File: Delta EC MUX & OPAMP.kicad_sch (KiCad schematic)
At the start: 32 parts, among them U6 OPA2365, U7 4052, U8 OPA2365, U9 4052

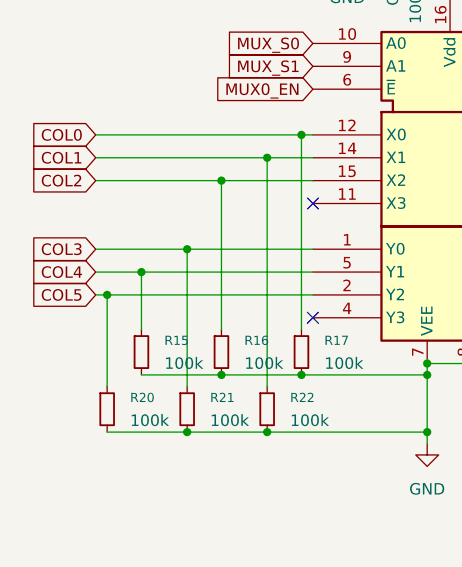
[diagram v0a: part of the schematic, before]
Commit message: 17.04.2026
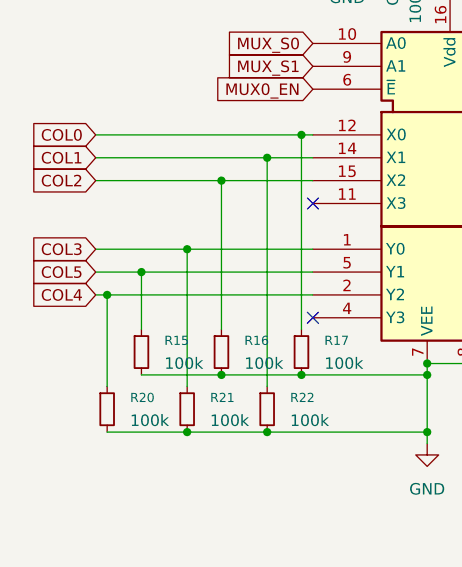
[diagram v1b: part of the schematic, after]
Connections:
- net COL4: now also R20.1, U7.2 (Y2); no longer R15.1, U7.5 (Y1)
- net COL5: now also R15.1, U7.5 (Y1); no longer R20.1, U7.2 (Y2)
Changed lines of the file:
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@@
 	(global_label "COL4"
 		(shape input)
+		(at 40.64 74.93 180)
+		(fields_autoplaced yes)
+		(effects
+			(font
+				(size 1.27 1.27)
+			)
+			(justify right)
+		)
+		(property "Intersheetrefs" "${INTERSHEET_REFS}"
+			(at 32.8167 74.93 0)
+			(effects
+				(font
+					(size 1.27 1.27)
+				)
+				(justify right)
+				(hide yes)
+			)
+		)
+	)
+	(global_label "COL3"
+		(shape input)
+		(at 40.64 69.85 180)
+		(fields_autoplaced yes)
+		(effects
+			(font
+				(size 1.27 1.27)
+			)
+			(justify right)
+		)
+		(property "Intersheetrefs" "${INTERSHEET_REFS}"
+			(at 32.8167 69.85 0)
+			(effects
+				(font
+					(size 1.27 1.27)
+				)
+				(justify right)
+				(hide yes)
+			)
+		)
+	)
+	(global_label "ADC2_IN"
+		(shape input)
+		(at 139.7 132.08 0)
+		(fields_autoplaced yes)
+		(effects
+			(font
+				(size 1.27 1.27)
+			)
+			(justify left)
+		)
+		(property "Intersheetrefs" "${INTERSHEET_REFS}"
+			(at 150.4262 132.08 0)
+			(effects
+				(font
+					(size 1.27 1.27)
+				)
+				(justify left)
+				(hide yes)
+			)
+		)
+	)
+	(global_label "ADC1_IN"
+		(shape input)
+		(at 119.38 76.2 0)
+		(fields_autoplaced yes)
+		(effects
+			(font
+				(size 1.27 1.27)
+			)
+			(justify left)
+		)
+		(property "Intersheetrefs" "${INTERSHEET_REFS}"
+			(at 130.1062 76.2 0)
+			(effects
+				(font
+					(size 1.27 1.27)
+				)
+				(justify left)
+				(hide yes)
+			)
+		)
+	)
+	(global_label "COL10"
+		(shape input)
+		(at 48.26 157.48 180)
+		(fields_autoplaced yes)
+		(effects
+			(font
+				(size 1.27 1.27)
+			)
+			(justify right)
+		)
+		(property "Intersheetrefs" "${INTERSHEET_REFS}"
+			(at 39.2272 157.48 0)
+			(effects
+				(font
+					(size 1.27 1.27)
+				)
+				(justify right)
+				(hide yes)
+			)
+		)
+	)
+	(global_label "COL1"
+		(shape input)
+		(at 40.64 59.69 180)
+		(fields_autoplaced yes)
+		(effects
+			(font
+				(size 1.27 1.27)
+			)
+			(justify right)
+		)
+		(property "Intersheetrefs" "${INTERSHEET_REFS}"
+			(at 32.8167 59.69 0)
+			(effects
+				(font
+					(size 1.27 1.27)
+				)
+				(justify right)
+				(hide yes)
+			)
+		)
+	)
+	(global_label "DISCHARGE0"
+		(shape input)
+		(at 104.14 43.18 90)
+		(fields_autoplaced yes)
+		(effects
+			(font
+				(size 1.27 1.27)
+			)
+			(justify left)
+		)
+		(property "Intersheetrefs" "${INTERSHEET_REFS}"
+			(at 104.14 28.5229 90)
+			(effects
+				(font
+					(size 1.27 1.27)
+				)
+				(justify left)
+				(hide yes)
+			)
+		)
+	)
+	(global_label "COL7"
+		(shape input)
+		(at 48.26 144.78 180)
+		(fields_autoplaced yes)
+		(effects
+			(font
+				(size 1.27 1.27)
+			)
+			(justify right)
+		)
+		(property "Intersheetrefs" "${INTERSHEET_REFS}"
+			(at 40.4367 144.78 0)
+			(effects
+				(font
+					(size 1.27 1.27)
+				)
+				(justify right)
+				(hide yes)
+			)
+		)
+	)
+	(global_label "MUX_S1"
+		(shape input)
+		(at 64.77 49.53 180)
+		(fields_autoplaced yes)
+		(effects
+			(font
+				(size 1.27 1.27)
+			)
+			(justify right)
+		)
+		(property "Intersheetrefs" "${INTERSHEET_REFS}"
+			(at 54.4068 49.53 0)
+			(effects
+				(font
+					(size 1.27 1.27)
+				)
+				(justify right)
+				(hide yes)
+			)
+		)
+	)
+	(global_label "DISCHARGE2"
+		(shape input)
+		(at 111.76 128.27 90)
+		(fields_autoplaced yes)
+		(effects
+			(font
+				(size 1.27 1.27)
+			)
+			(justify left)
+		)
+		(property "Intersheetrefs" "${INTERSHEET_REFS}"
+			(at 111.76 113.6129 90)
+			(effects
+				(font
+					(size 1.27 1.27)
+				)
+				(justify left)
+				(hide yes)
+			)
+		)
+	)
+	(global_label "DISCHARGE3"
+		(shape input)
+		(at 105.41 157.48 90)
+		(fields_autoplaced yes)
+		(effects
+			(font
+				(size 1.27 1.27)
+			)
+			(justify left)
+		)
+		(property "Intersheetrefs" "${INTERSHEET_REFS}"
+			(at 105.41 142.8229 90)
+			(effects
+				(font
+					(size 1.27 1.27)
+				)
+				(justify left)
+				(hide yes)
+			)
+		)
+	)
+	(global_label "COL5"
+		(shape input)
 		(at 40.64 72.39 180)
 		(fields_autoplaced yes)
@@
 			(effects
 				(font
-					(size 1.27 1.27)
-				)
-				(justify right)
-				(hide yes)
-			)
-		)
-	)
-	(global_label "COL3"
-		(shape input)
-		(at 40.64 69.85 180)
-		(fields_autoplaced yes)
-		(effects
-			(font
-				(size 1.27 1.27)
-			)
-			(justify right)
-		)
-		(property "Intersheetrefs" "${INTERSHEET_REFS}"
-			(at 32.8167 69.85 0)
-			(effects
-				(font
-					(size 1.27 1.27)
-				)
-				(justify right)
-				(hide yes)
-			)
-		)
-	)
-	(global_label "ADC2_IN"
-		(shape input)
-		(at 139.7 132.08 0)
-		(fields_autoplaced yes)
-		(effects
-			(font
-				(size 1.27 1.27)
-			)
-			(justify left)
-		)
-		(property "Intersheetrefs" "${INTERSHEET_REFS}"
-			(at 150.4262 132.08 0)
-			(effects
-				(font
-					(size 1.27 1.27)
-				)
-				(justify left)
-				(hide yes)
-			)
-		)
-	)
-	(global_label "ADC1_IN"
-		(shape input)
-		(at 119.38 76.2 0)
-		(fields_autoplaced yes)
-		(effects
-			(font
-				(size 1.27 1.27)
-			)
-			(justify left)
-		)
-		(property "Intersheetrefs" "${INTERSHEET_REFS}"
-			(at 130.1062 76.2 0)
-			(effects
-				(font
-					(size 1.27 1.27)
-				)
-				(justify left)
-				(hide yes)
-			)
-		)
-	)
-	(global_label "COL10"
-		(shape input)
-		(at 48.26 157.48 180)
-		(fields_autoplaced yes)
-		(effects
-			(font
-				(size 1.27 1.27)
-			)
-			(justify right)
-		)
-		(property "Intersheetrefs" "${INTERSHEET_REFS}"
-			(at 39.2272 157.48 0)
-			(effects
-				(font
-					(size 1.27 1.27)
-				)
-				(justify right)
-				(hide yes)
-			)
-		)
-	)
-	(global_label "COL1"
-		(shape input)
-		(at 40.64 59.69 180)
-		(fields_autoplaced yes)
-		(effects
-			(font
-				(size 1.27 1.27)
-			)
-			(justify right)
-		)
-		(property "Intersheetrefs" "${INTERSHEET_REFS}"
-			(at 32.8167 59.69 0)
-			(effects
-				(font
-					(size 1.27 1.27)
-				)
-				(justify right)
-				(hide yes)
-			)
-		)
-	)
-	(global_label "DISCHARGE0"
-		(shape input)
-		(at 104.14 43.18 90)
-		(fields_autoplaced yes)
-		(effects
-			(font
-				(size 1.27 1.27)
-			)
-			(justify left)
-		)
-		(property "Intersheetrefs" "${INTERSHEET_REFS}"
-			(at 104.14 28.5229 90)
-			(effects
-				(font
-					(size 1.27 1.27)
-				)
-				(justify left)
-				(hide yes)
-			)
-		)
-	)
-	(global_label "COL7"
-		(shape input)
-		(at 48.26 144.78 180)
-		(fields_autoplaced yes)
-		(effects
-			(font
-				(size 1.27 1.27)
-			)
-			(justify right)
-		)
-		(property "Intersheetrefs" "${INTERSHEET_REFS}"
-			(at 40.4367 144.78 0)
-			(effects
-				(font
-					(size 1.27 1.27)
-				)
-				(justify right)
-				(hide yes)
-			)
-		)
-	)
-	(global_label "MUX_S1"
-		(shape input)
-		(at 64.77 49.53 180)
-		(fields_autoplaced yes)
-		(effects
-			(font
-				(size 1.27 1.27)
-			)
-			(justify right)
-		)
-		(property "Intersheetrefs" "${INTERSHEET_REFS}"
-			(at 54.4068 49.53 0)
-			(effects
-				(font
-					(size 1.27 1.27)
-				)
-				(justify right)
-				(hide yes)
-			)
-		)
-	)
-	(global_label "DISCHARGE2"
-		(shape input)
-		(at 111.76 128.27 90)
-		(fields_autoplaced yes)
-		(effects
-			(font
-				(size 1.27 1.27)
-			)
-			(justify left)
-		)
-		(property "Intersheetrefs" "${INTERSHEET_REFS}"
-			(at 111.76 113.6129 90)
-			(effects
-				(font
-					(size 1.27 1.27)
-				)
-				(justify left)
-				(hide yes)
-			)
-		)
-	)
-	(global_label "DISCHARGE3"
-		(shape input)
-		(at 105.41 157.48 90)
-		(fields_autoplaced yes)
-		(effects
-			(font
-				(size 1.27 1.27)
-			)
-			(justify left)
-		)
-		(property "Intersheetrefs" "${INTERSHEET_REFS}"
-			(at 105.41 142.8229 90)
-			(effects
-				(font
-					(size 1.27 1.27)
-				)
-				(justify left)
-				(hide yes)
-			)
-		)
-	)
-	(global_label "COL5"
-		(shape input)
-		(at 40.64 74.93 180)
-		(fields_autoplaced yes)
-		(effects
-			(font
-				(size 1.27 1.27)
-			)
-			(justify right)
-		)
-		(property "Intersheetrefs" "${INTERSHEET_REFS}"
-			(at 32.8167 74.93 0)
-			(effects
-				(font
